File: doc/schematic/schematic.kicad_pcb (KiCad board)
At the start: 2 copper layers, 11 parts, among them J1 TFT_Power, J15 fz35, J18 USB, J19 Switch, J3 TFT, J7 INA, U1 ESP32-S3-DevKitC

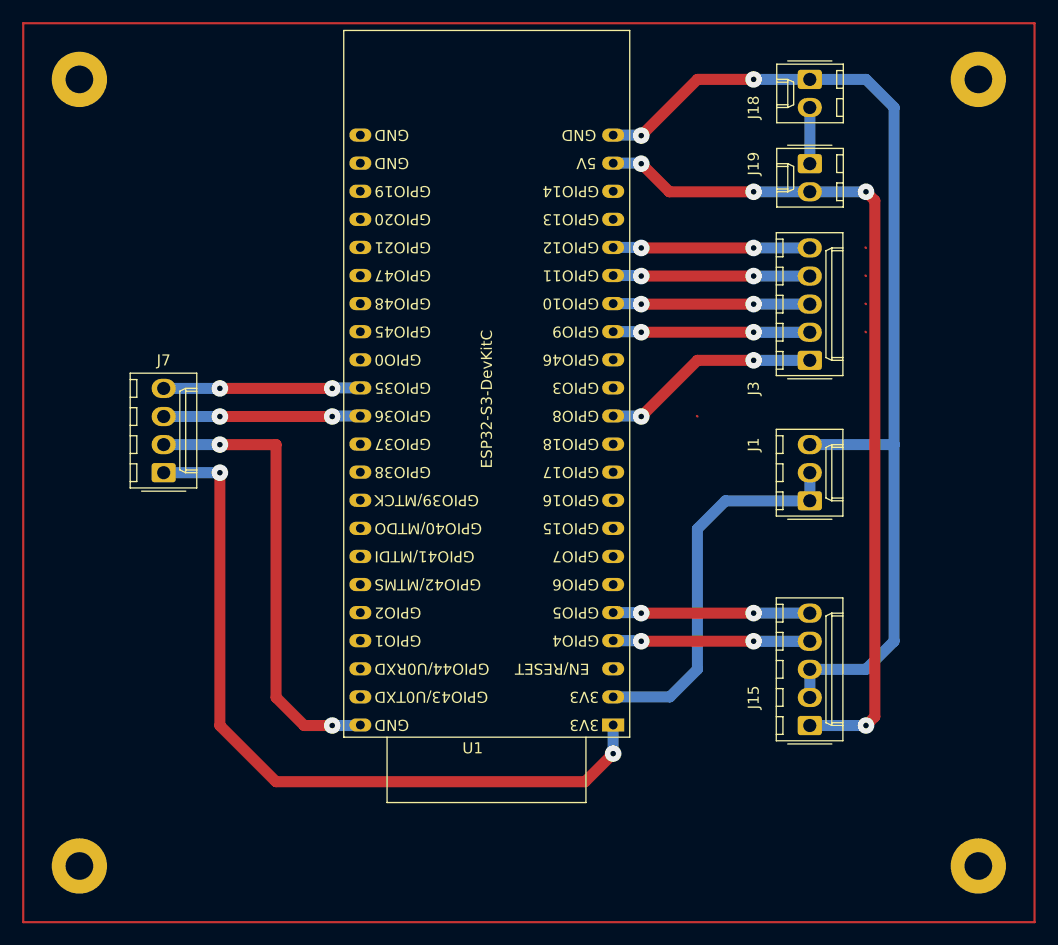
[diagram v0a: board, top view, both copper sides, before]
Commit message: full functionality
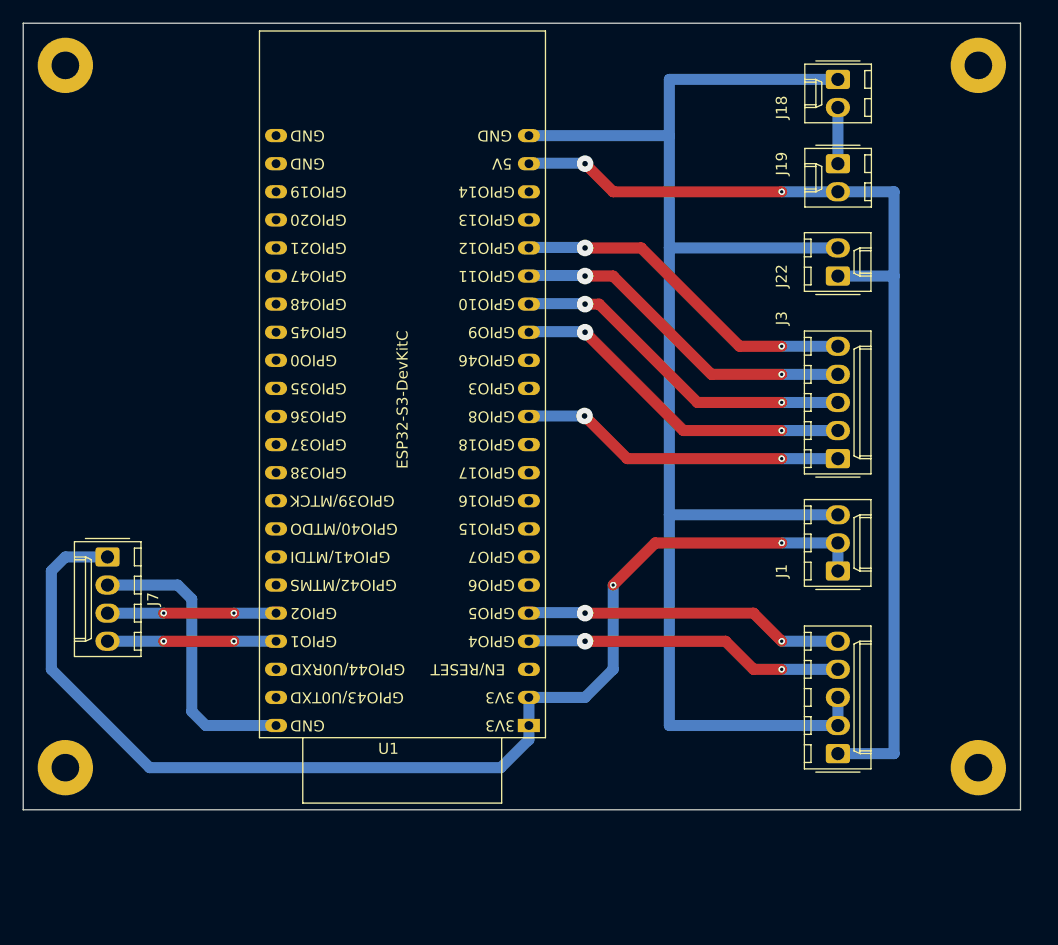
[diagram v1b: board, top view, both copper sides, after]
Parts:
- added J22: Fan, Connector_Molex:Molex_KK-254_AE-6410-02A_1x02_P2.54mm_Vertical, F.Cu at (142.2, 73.7)
- moved J3 9.25 mm to (142.2, 90.2)
- moved J7 9.16 mm to (76.2, 99.1), turned to -90 degrees
- moved REF** 8.98 mm to (72.4, 118.1)
- moved REF** 8.89 mm to (154.9, 118.1)
- moved U1 7.62 mm to (114.3, 114.3)
- moved J1 6.84 mm to (142.2, 100.3)
- moved J15 3.59 mm to (142.2, 116.8)
- moved J18 2.54 mm to (142.2, 55.9)
- moved J19 2.54 mm to (142.2, 63.5)
- moved REF** 1.80 mm to (72.4, 54.6)
- moved REF** 1.27 mm to (154.9, 54.6)
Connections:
- U1 pad 23: GND -> unconnected-(U1-GND-Pad23)
- U1 pad 24: GND -> unconnected-(U1-GND-Pad24)
- U1 pad 32: Net-(J7-Pin_4) -> unconnected-(U1-GPIO35-Pad32)
- U1 pad 33: Net-(J7-Pin_3) -> unconnected-(U1-GPIO36-Pad33)
- U1 pad 40: unconnected-(U1-GPIO2/ADC1_CH1-Pad40) -> Net-(J7-Pin_3)
- U1 pad 41: unconnected-(U1-GPIO1/ADC1_CH0-Pad41) -> Net-(J7-Pin_4)
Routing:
- net GND: track 137.4 -> 161.1 mm, vias 4 -> 0
- net +5V: track 77.9 -> 95.1 mm, vias 4 -> 2
- net Net-(J3-Pin_5): track 17.9 -> 31.7 mm
- net Net-(J3-Pin_3): track 17.9 -> 31.7 mm
- net Net-(J3-Pin_4): track 17.9 -> 31.7 mm
- net Net-(J3-Pin_2): track 17.9 -> 31.7 mm
- net Net-(J15-Pin_5): track 17.8 -> 29.0 mm
- net Net-(J15-Pin_4): track 17.8 -> 29.0 mm
- net Net-(J3-Pin_1): track 20.0 -> 29.6 mm
- net +3V3: track 104.3 -> 107.0 mm
- net Net-(J7-Pin_3): track 17.8 -> 15.2 mm
- net Net-(J7-Pin_4): track 17.8 -> 15.2 mm
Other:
- board outline added: 90.2 x 71.1 mm
